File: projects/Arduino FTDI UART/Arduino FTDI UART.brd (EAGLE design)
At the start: 48.3 x 30.5 mm, 18 parts, among them IC1 FT232RL, X1 MINI-USB-32005-201

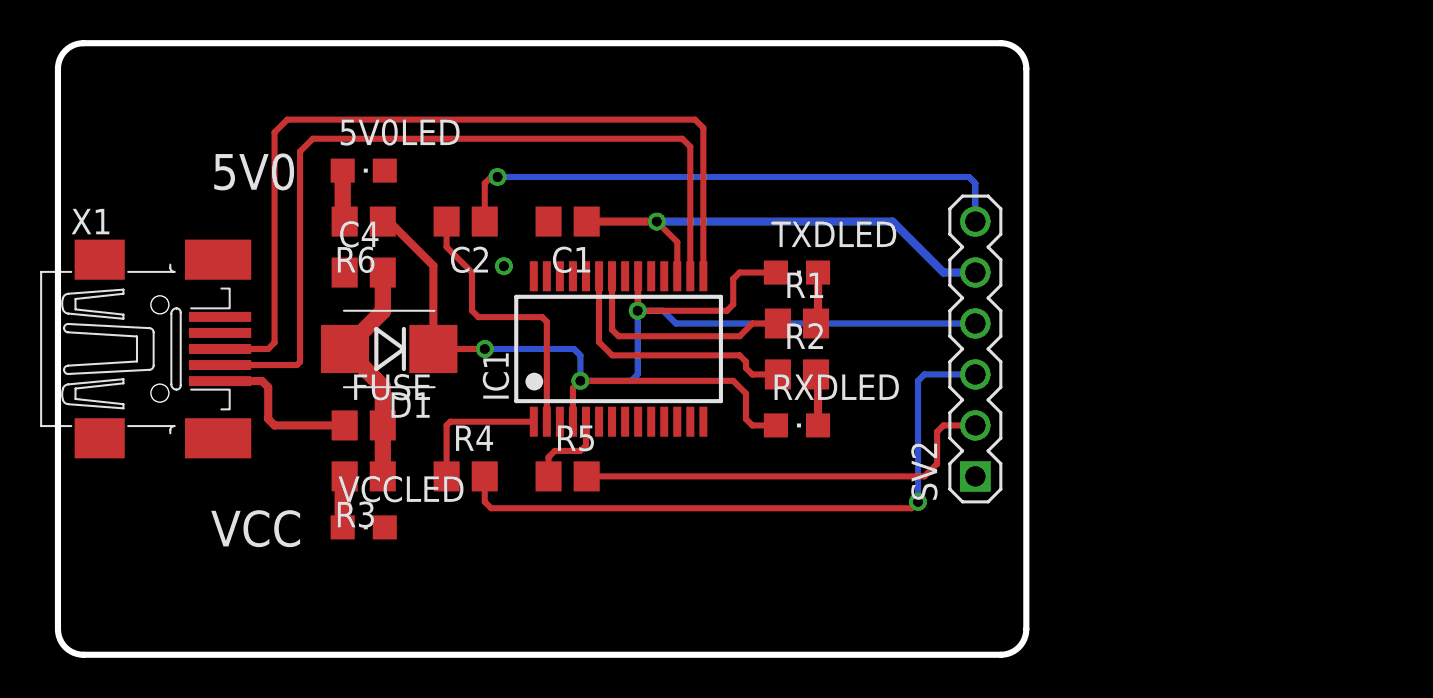
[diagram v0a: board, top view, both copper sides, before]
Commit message: 2020.05.25.01
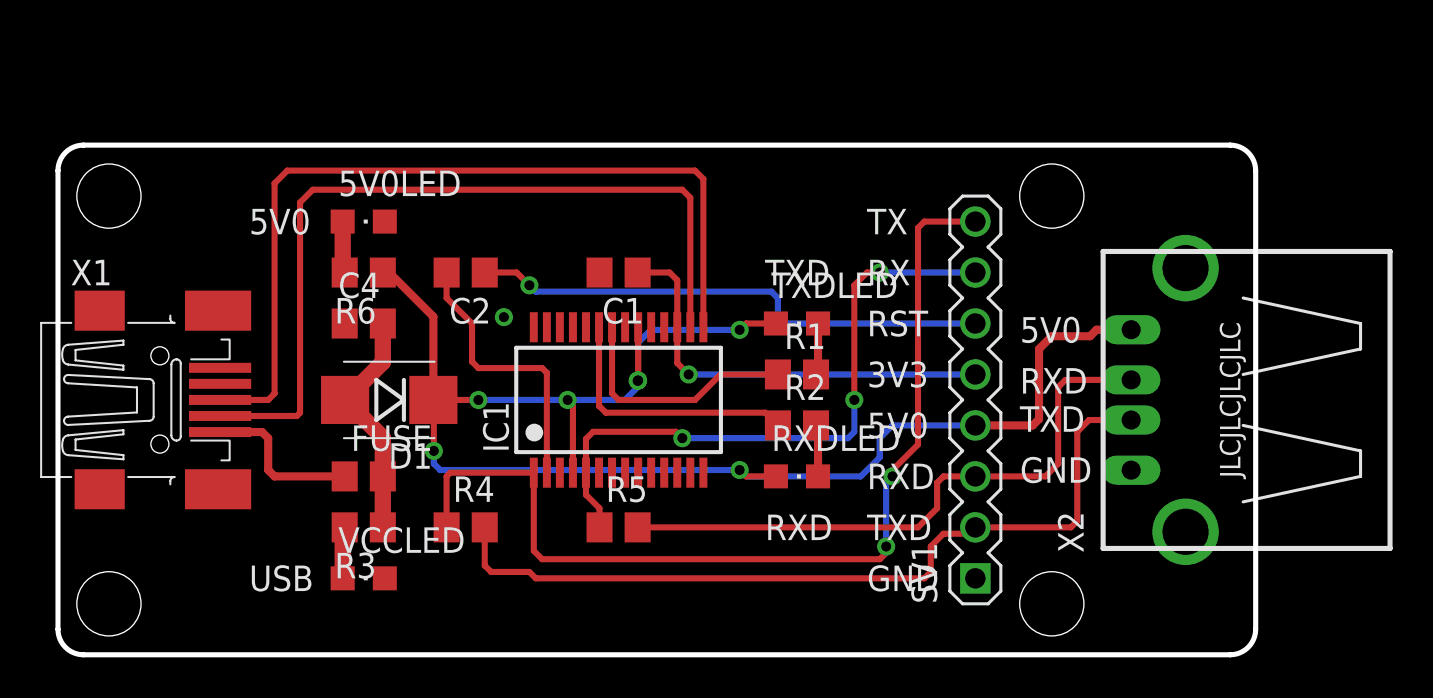
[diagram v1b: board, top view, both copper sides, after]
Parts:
- removed SV2: (no value), Pin-Header:MA06-1
- added SV1: (no value), Pin-Header:MA08-1
- added X2: USB-A-SHIELD, Socket:USB-A-SHIELD
- X1: value MINI-USB-32005-201 -> MINI-USB
- moved R5 3.59 mm to (27.9, 6.35)
- moved C1 3.59 mm to (27.9, 19.1)
- moved D1 2.54 mm to (16.5, 12.7)
- moved IC1 2.54 mm to (27.9, 12.7)
- moved R1 2.54 mm to (36.8, 14.0)
- moved R2 2.54 mm to (36.8, 11.4)
- moved R3 2.54 mm to (15.2, 6.35)
- moved R4 2.54 mm to (20.3, 6.35)
- moved X1 2.54 mm to (5.08, 12.7)
- moved VCCLED 2.54 mm to (15.2, 3.81)
- moved 5V0LED 2.54 mm to (15.2, 21.6)
- moved C2 2.54 mm to (20.3, 19.1)
- moved C4 2.54 mm to (15.2, 16.5)
- moved FUSE 2.54 mm to (15.2, 8.89)
- moved R6 2.54 mm to (15.2, 19.1)
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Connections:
- removed net N$2: IC1.1, R4.1
- removed net N$8: IC1.5, R5.1
- new net RX: IC1.5, R5.1, SV1.7
- new net TX: IC1.1, R4.1, SV1.8
- net +3V3: now also SV1.5; no longer SV2.5
- net +5V: now also SV1.4, X2.4; no longer SV2.4
- net GND: now also SV1.1, X2.1, X2.S1, X2.S2; no longer SV2.1
- net RESET: now also SV1.6; no longer SV2.6
- net RXD: now also SV1.3, X2.3; no longer SV2.2
- net TXD: now also SV1.2, X2.2; no longer SV2.3
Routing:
- net TX: track 0.00 -> 48.6 mm, vias 0 -> 2
- net RX: track 0.00 -> 32.1 mm, vias 0 -> 3
- net +5V: track 65.0 -> 79.7 mm, vias 3 -> 6
- net RXD: track 21.4 -> 30.6 mm
- net TXD: track 32.1 -> 41.0 mm, vias 1 -> 0
- net N$2: track 6.97 -> 0.00 mm, vias 0 -> 1
- net N$8: track 4.24 -> 0.00 mm
- net RESET: track 28.5 -> 26.1 mm
- net +3V3: track 23.6 -> 21.4 mm
- net TXDLED: track 11.3 -> 12.2 mm
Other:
- board size 48.3 x 30.5 mm -> 59.7 x 25.4 mm
- board text added: "3V3"
- board text added: "Designed by DIOSTUDIO"
- board text added: "GND"
- board text added: "JLCJLCJLCJLC"
- board text added: "RST"
- board text added: "RX"
- board text added: "RXD"
- board text added: "TX"
- board text added: "TXD"
- board text added: "USB"
- board text added: "www.diostudio.cn"
- board text removed: "VCC"

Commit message: 2020.05.27.01
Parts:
- R1, R2: value 102 -> 331
- R3, R6: value 102 -> 471
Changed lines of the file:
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@@
 <element name="VCCLED" library="Display" package="CHIPLED_0805" value="RED" x="15.24" y="3.81" rot="R270"/>
 <element name="C1" library="RCLDA" package="C0805" value="104" x="27.94" y="19.05" rot="R180"/>
-<element name="R1" library="RCLDA" package="R0805" value="102" x="36.83" y="13.97"/>
+<element name="R1" library="RCLDA" package="R0805" value="331" x="36.83" y="13.97"/>
 <element name="D1" library="RCLDA" package="SMB" value="DIODESMB" x="16.51" y="12.7" rot="R180"/>
 <element name="X1" library="Socket" package="32005-201" value="MINI-USB" x="5.08" y="12.7">
@@
 </element>
 <element name="FUSE" library="RCLDA" package="R0805" value="" x="15.24" y="8.89"/>
-<element name="R2" library="RCLDA" package="R0805" value="102" x="36.83" y="11.43"/>
-<element name="R3" library="RCLDA" package="R0805" value="102" x="15.24" y="6.35" rot="R180"/>
+<element name="R2" library="RCLDA" package="R0805" value="331" x="36.83" y="11.43"/>
+<element name="R3" library="RCLDA" package="R0805" value="471" x="15.24" y="6.35" rot="R180"/>
 <element name="C2" library="RCLDA" package="C0805" value="104" x="20.32" y="19.05" rot="R180"/>
 <element name="C4" library="RCLDA" package="C0805" value="104" x="15.24" y="16.51"/>
 <element name="R4" library="RCLDA" package="R0805" value="102" x="20.32" y="6.35"/>
 <element name="R5" library="RCLDA" package="R0805" value="102" x="27.94" y="6.35"/>
-<element name="R6" library="RCLDA" package="R0805" value="102" x="15.24" y="19.05" rot="R180"/>
+<element name="R6" library="RCLDA" package="R0805" value="471" x="15.24" y="19.05" rot="R180"/>
 <element name="5V0LED" library="Display" package="CHIPLED_0805" value="RED" x="15.24" y="21.59" rot="R270"/>
 <element name="X2" library="Socket" package="USB-A-SHIELD" value="USB-A-SHIELD" x="56.1975" y="12.7" rot="R90">
